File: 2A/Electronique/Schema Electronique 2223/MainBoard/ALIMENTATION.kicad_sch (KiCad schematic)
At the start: 14 parts, among them Q3 PMOS, U1 TSR_1-2450

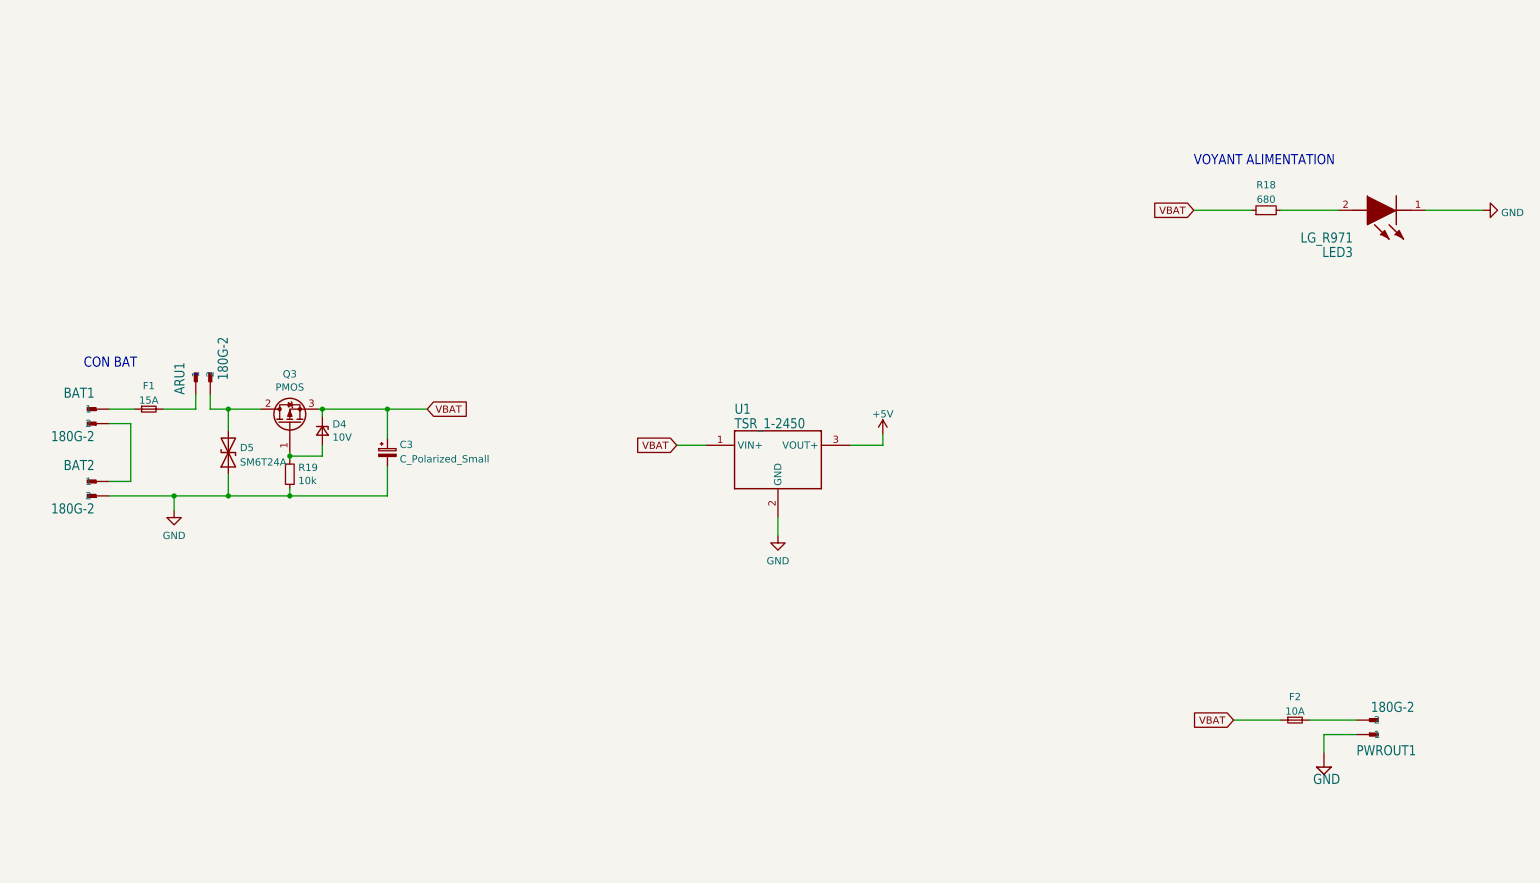
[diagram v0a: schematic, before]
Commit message: schematic and pcb update, added BOM
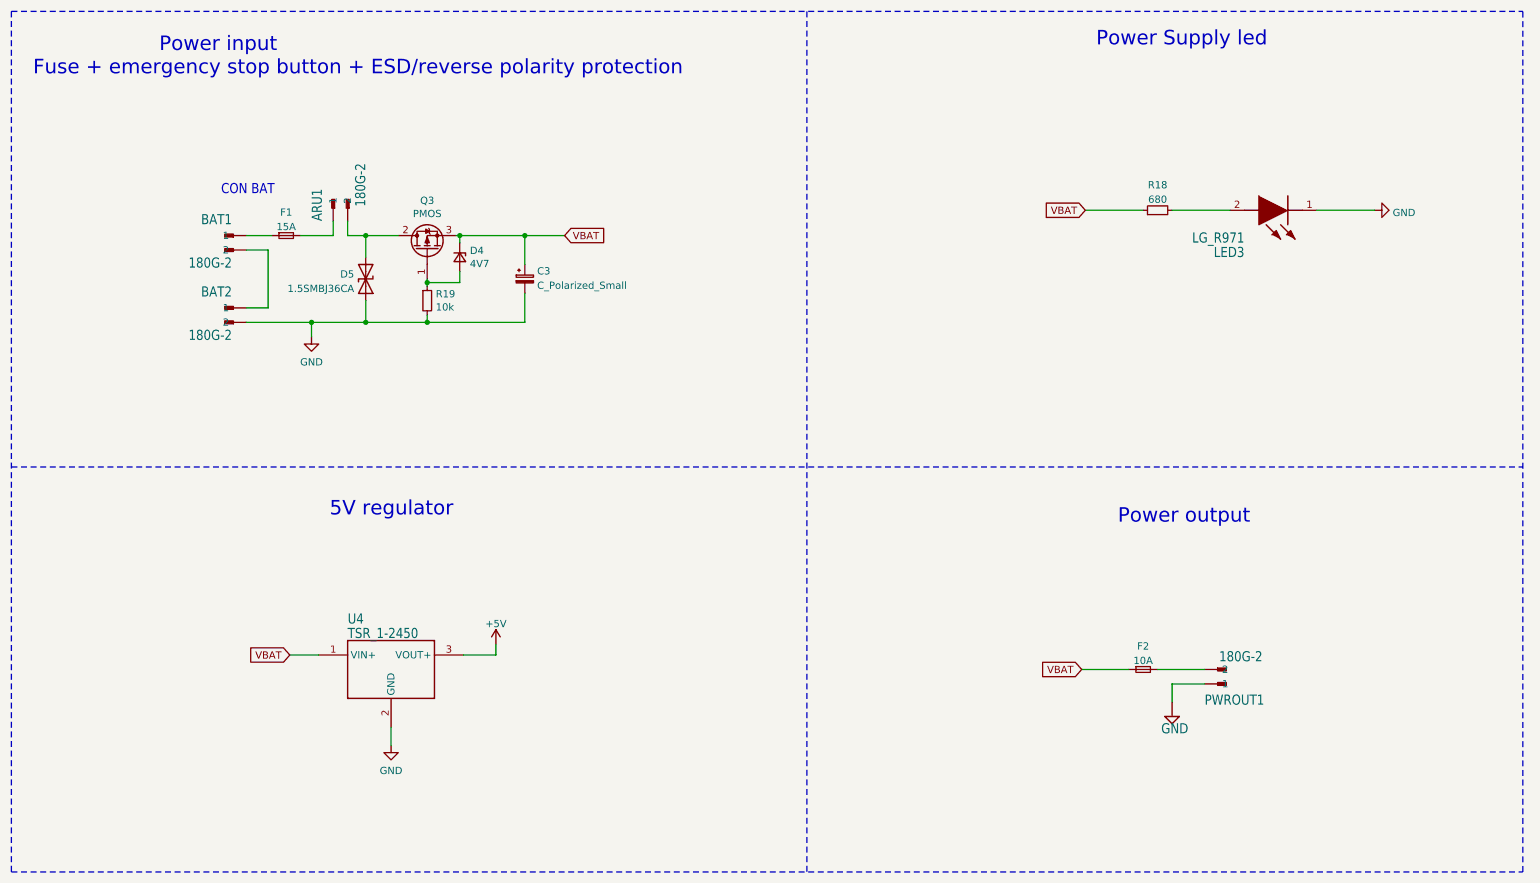
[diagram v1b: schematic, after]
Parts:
- D4: value 10V -> 4V7; Mouser Part Number (none) -> 771-BZX84J-C4V7115
- D5: value SM6T24A -> 1.5SMBJ36CA; Mouser Part Number (none) -> 652-1.5SMBJ36CA-H
- F1: Mouser Part Number (none) -> 693-3413.0330.22
- F2: Mouser Part Number (none) -> 530-0685P9100-01
- Q3: Mouser Part Number (none) -> 863-NTTFS015P03P8ZWG
- renumbered U1 to U4
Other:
- note added: "5V regulator"
- note added: "Power Supply led"
- note added: "Power input Fuse + emergency stop button + ESD/reverse polarity protection"
- note added: "Power output"
- note removed: "VOYANT ALIMENTATION"
- moved on the sheet: ARU1, BAT1, BAT2, C3, D4, D5, F1, F2, LED3, PWROUT1, Q3, R18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
